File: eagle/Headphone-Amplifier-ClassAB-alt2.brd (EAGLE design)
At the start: 17 parts, among them T1 BC547, T2 BC327, T3 BC337

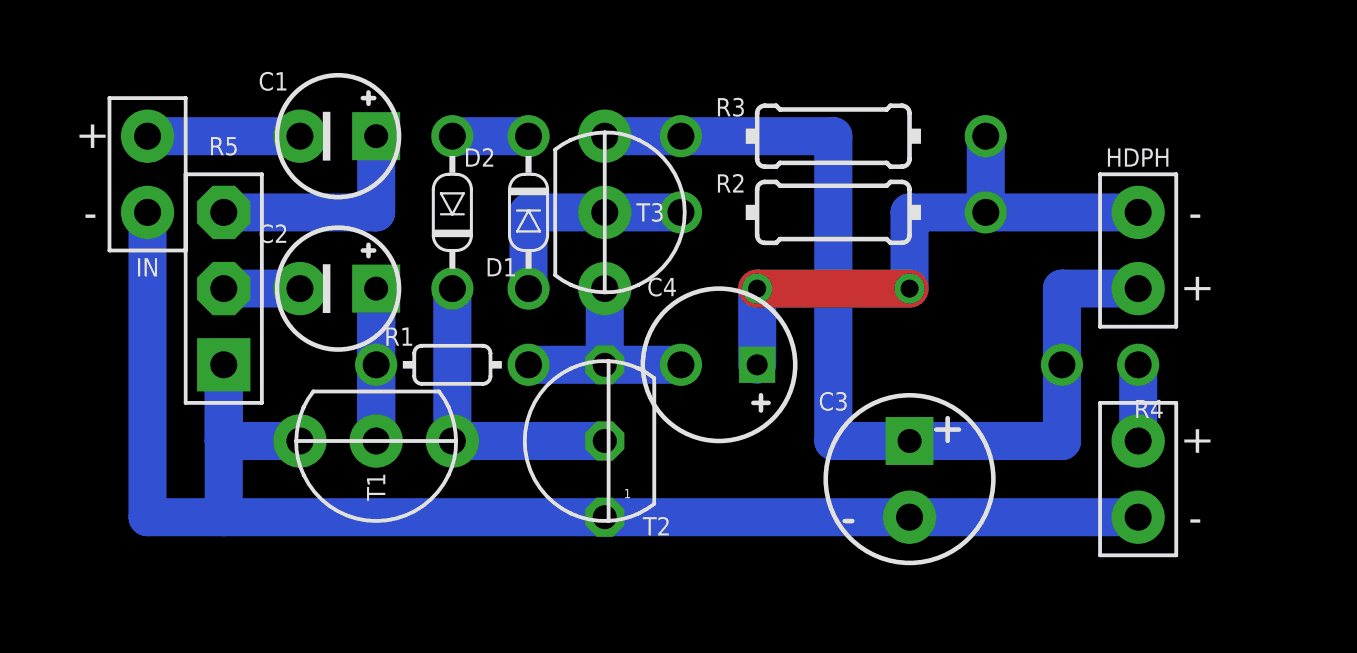
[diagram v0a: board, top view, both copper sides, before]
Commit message: ...
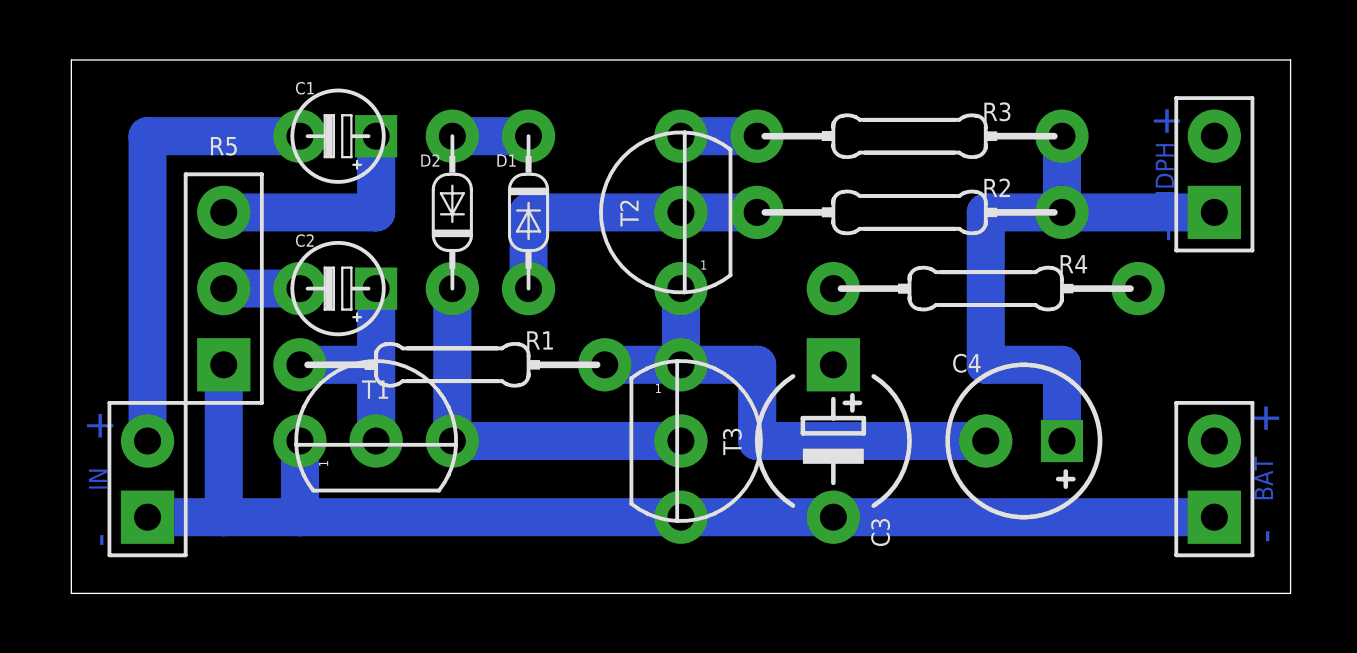
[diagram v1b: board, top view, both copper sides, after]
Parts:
- BAT: value (none) -> SPAD+-+-
- C1, C2: device c:E2,5-4 -> c:E2,5-3
- C3: value 100-1000uF -> 470uF; device c:E2,5-6/V -> c:E5-5
- C4: value 220uF -> 100uF
- D1: value (none) -> 1N4148; device d:DO34-5V -> d:DO34-5-V
- D2: value (none) -> 1N4148
- IN: value (none) -> SPAD+--+
- R1: device r:0202/5 -> r:0204/10
- R4: value 22 -> 27; device r:0204/2.54 -> r:0204/10
- T1: value BC547 -> 2N3904; device t:TO92-CBE -> t:TO92
- T2: value BC327 -> 2N3904
- T3: value BC337 -> 2N3906; device t:TO92-CBE -> t:TO92
- moved C4 10.5 mm to (31.8, 5.08)
- moved IN 10.2 mm to (2.54, 3.81)
- moved T2 8.03 mm to (20.3, 12.7)
- moved T3 8.03 mm to (20.3, 5.08)
- moved R4 4.58 mm to (30.5, 10.2), turned to 0 degrees
- moved HDPH 3.59 mm to (38.1, 14.0), turned to 0 degrees
- moved C3 2.84 mm to (25.4, 5.08), turned to 270 degrees
- moved R2 2.54 mm to (27.9, 12.7)
- moved R3 2.54 mm to (27.9, 15.2)
- moved BAT 2.54 mm to (38.1, 3.81)
- turned C1 to 180 degrees
- turned C2 to 180 degrees
- turned D1 to 0 degrees
- turned T1 to 90 degrees
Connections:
- net GND: now also T1.1, T3.3; no longer T1.E, T2.1
- net N$1: now also T2.2; no longer T3.B
- net N$2: now also T1.3, T3.2; no longer T1.C, T2.2
- net N$4: now also T2.1, T3.1; no longer T2.3, T3.E
- net N$7: now also T1.2; no longer T1.B
- net N$8: now also T2.3; no longer T3.C
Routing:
- net N$8: track 33.0 -> 2.54 mm
- net GND: track 53.3 -> 43.2 mm
- net N$4: track 7.62 -> 17.8 mm
- net N$10: track 5.08 -> 15.2 mm
- net N$6: track 7.62 -> 2.54 mm
- net V+: track 2.54 -> 0.00 mm
- net N$7: track 5.08 -> 7.62 mm
- net N$2: track 10.2 -> 12.7 mm
- net N$1: track 7.62 -> 10.2 mm
- net N$9: vias 2 -> 0
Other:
- board outline added: 40.6 x 17.8 mm
